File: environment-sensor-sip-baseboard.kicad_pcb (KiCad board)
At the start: 4 copper layers, 50 x 26.5 mm, 60 parts, among them J1 USB-C_GCT_USB4105-GF-A, J2 JST_SH_1x4_SM04B-SRSS-TB-LF-SN, J3 JST_SH_1x4_SM04B-SRSS-TB-LF-SN, U1 Antmicro_GEM3, U5 SHT45, U6 BME280

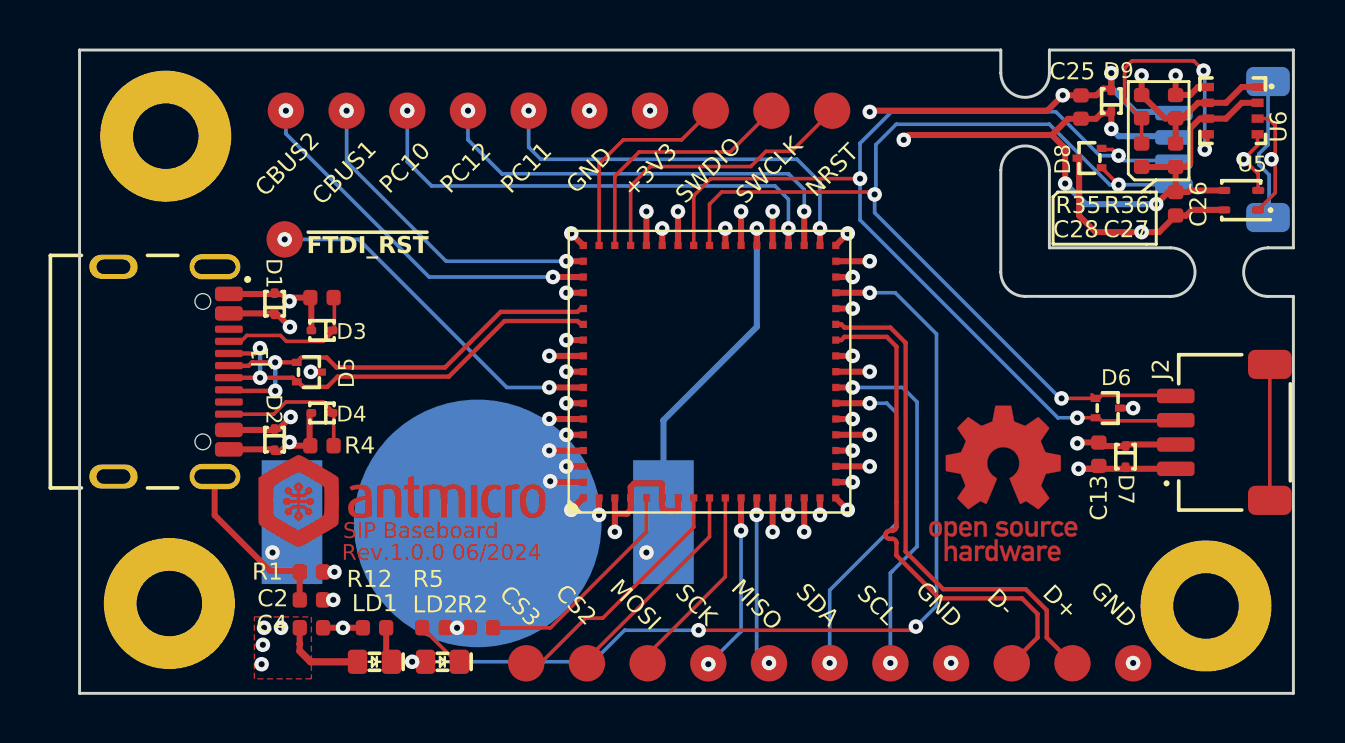
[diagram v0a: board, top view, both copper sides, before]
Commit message: [#61553] Update title block
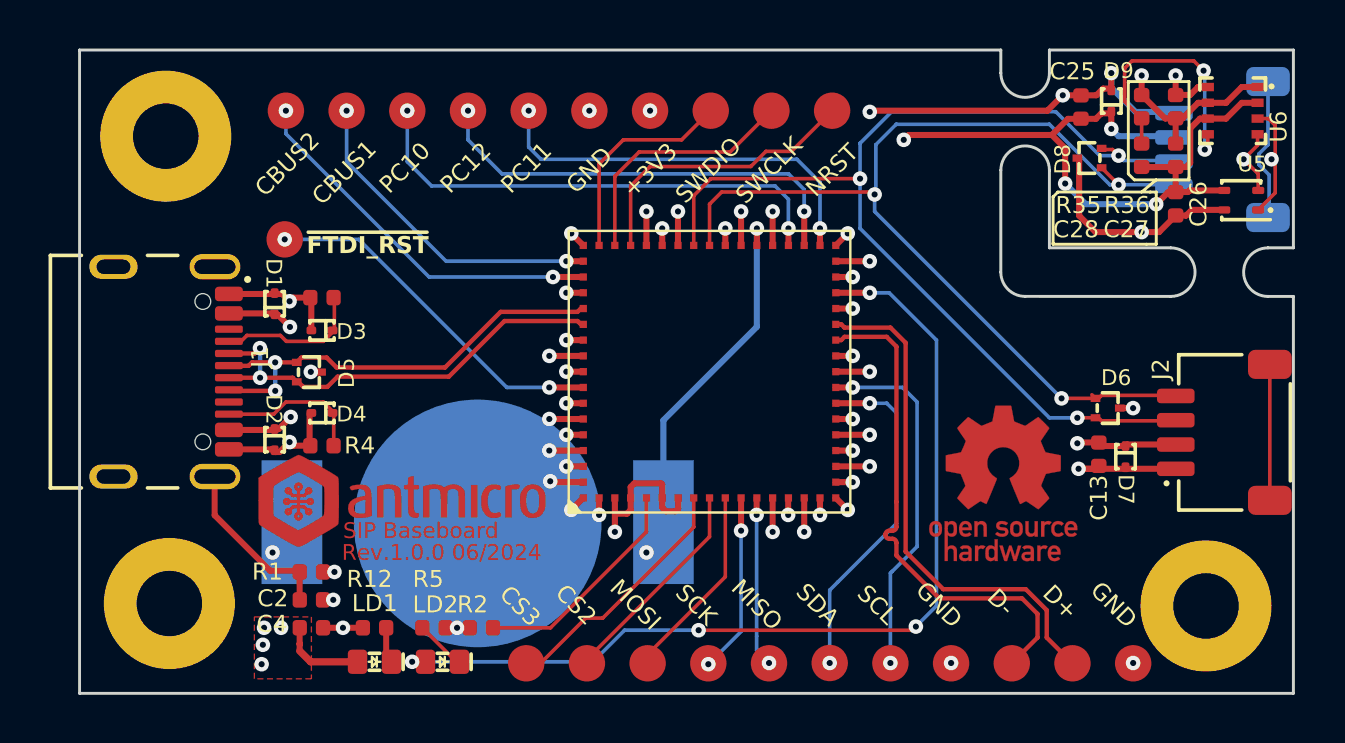
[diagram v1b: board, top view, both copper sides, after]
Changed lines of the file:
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@@
   )
   (paper "A4")
+  (title_block
+    (title "SiP Baseboard")
+    (date "2024-06-28")
+    (rev "1.0.0")
+    (company "Antmicro ")
+    (comment 1 "www.antmicro.com")
+  )
   (layers
     (0 "F.Cu" signal)
@@
     (tags "resistor SMD 0402")
     (property "Author" "Antmicro")
-    (property "DNP" "DNP")
     (property "License" "Apache-2.0")
     (property "MPN" "CR0402-FX-5101GLF")
@@
     (property "ki_description" "SMD Chip Resistor, 5.1 kohm, ± 1%, 63 mW, 0402 [1005 Metric], Thick Film, General Purpose")
     (property "ki_keywords" "0402, SMT, RESISTOR, PASSIVE")
-    (attr smd exclude_from_pos_files exclude_from_bom)
+    (attr smd)
     (fp_text reference "R2" (at -1 -0.55) (layer "F.SilkS")
         (effects (font (size 0.7 0.7) (thickness 0.15)) (justify left bottom))
@@
     (property "ki_description" "SMD Chip Resistor, 100 kohm, ± 1%, 62.5 mW, 0402 [1005 Metric], Thick Film, General Purpose")
     (property "ki_keywords" "0402, SMT, RESISTOR, PASSIVE")
-    (attr smd exclude_from_pos_files exclude_from_bom)
+    (attr smd)
     (fp_text reference "R35" (at -2.465 -3.55 180) (layer "F.SilkS")
         (effects (font (size 0.7 0.7) (thickness 0.15)) (justify left bottom))
@@
     (property "ki_description" "SMD Chip Resistor, 1 Mohm, ± 1%, 62.5 mW, 0402 [1005 Metric], Thick Film, General Purpose")
     (property "ki_keywords" "0402, SMT, RESISTOR, PASSIVE")
-    (attr smd exclude_from_pos_files exclude_from_bom)
+    (attr smd)
     (fp_text reference "R1" (at -2.45 0.4) (layer "F.SilkS")
         (effects (font (size 0.7 0.7) (thickness 0.15)) (justify left bottom))
@@
   (segment (start 207.825 118.125) (end 203.725 118.125) (width 0.15) (layer "In2.Cu") (net 9))
   (segment (start 203.725 118.125) (end 202.8 119.05) (width 0.15) (layer "In2.Cu") (net 9))
+  (segment (start 192.75 119.45) (end 192.75 120.15) (width 0.15) (layer "B.Cu") (net 9))
   (segment (start 193.642 116.558) (end 199.947 116.558) (width 0.15) (layer "B.Cu") (net 9))
-  (segment (start 192.75 119.45) (end 192.75 120.2) (width 0.15) (layer "B.Cu") (net 9))
   (segment (start 202.8 119.05) (end 204.8 119.05) (width 0.15) (layer "B.Cu") (net 9))
   (segment (start 192.8 117.4) (end 193.642 116.558) (width 0.15) (layer "B.Cu") (net 9))
   (segment (start 192.75 119.45) (end 192.8 119.4) (width 0.15) (layer "B.Cu") (net 9))
+  (segment (start 192.75 120.15) (end 200.45 127.85) (width 0.15) (layer "B.Cu") (net 9))
   (segment (start 202.439 119.05) (end 202.8 119.05) (width 0.15) (layer "B.Cu") (net 9))
   (segment (start 192.8 119.4) (end 192.8 117.4) (width 0.15) (layer "B.Cu") (net 9))
-  (segment (start 200.4 127.85) (end 200.45 127.85) (width 0.15) (layer "B.Cu") (net 9))
   (segment (start 199.947 116.558) (end 202.439 119.05) (width 0.15) (layer "B.Cu") (net 9))
-  (segment (start 192.75 120.2) (end 200.4 127.85) (width 0.15) (layer "B.Cu") (net 9))
   (segment (start 185.3 119.5) (end 186 118.8) (width 0.15) (layer "F.Cu") (net 10))
   (segment (start 202.025 117.6) (end 202.55 117.6) (width 0.15) (layer "F.Cu") (net 10))
@@
   (segment (start 209.1 118) (end 208.175 117.075) (width 0.15) (layer "In2.Cu") (net 10))
   (segment (start 203 118.05) (end 204.8 118.05) (width 0.15) (layer "B.Cu") (net 10))
+  (segment (start 192.15 120.85) (end 199.95 128.65) (width 0.15) (layer "B.Cu") (net 10))
   (segment (start 193.449463 116.043) (end 200.214 116.043) (width 0.15) (layer "B.Cu") (net 10))
   (segment (start 200.214 116.043) (end 202.021 117.85) (width 0.15) (layer "B.Cu") (net 10))
   (segment (start 192.15 117.342463) (end 193.449463 116.043) (width 0.15) (layer "B.Cu") (net 10))
   (segment (start 202.021 117.85) (end 202.8 117.85) (width 0.15) (layer "B.Cu") (net 10))
-  (segment (start 192.15 120.5) (end 200.3 128.65) (width 0.15) (layer "B.Cu") (net 10))
+  (segment (start 192.15 118.8) (end 192.15 120.85) (width 0.15) (layer "B.Cu") (net 10))
   (segment (start 202.8 117.85) (end 203 118.05) (width 0.15) (layer "B.Cu") (net 10))
   (segment (start 192.15 118.8) (end 192.15 117.342463) (width 0.15) (layer "B.Cu") (net 10))
-  (segment (start 192.15 118.8) (end 192.15 120.5) (width 0.15) (layer "B.Cu") (net 10))
-  (segment (start 200.3 128.65) (end 201.1 128.65) (width 0.15) (layer "B.Cu") (net 10))
+  (segment (start 199.95 128.65) (end 201.1 128.65) (width 0.15) (layer "B.Cu") (net 10))
   (segment (start 191.15 123.5) (end 192.549999 123.5) (width 0.25) (layer "F.Cu") (net 11))
   (segment (start 194.3 137.4) (end 185.5 137.4) (width 0.15) (layer "F.Cu") (net 11))
@@
   (segment (start 173.7 138.7) (end 181.15 138.7) (width 0.15) (layer "B.Cu") (net 11))
   (segment (start 182.45 137.4) (end 185.5 137.4) (width 0.15) (layer "B.Cu") (net 11))
-  (segment (start 193.6 123.5) (end 192.549999 123.5) (width 0.15) (layer "B.Cu") (net 11))
-  (segment (start 195.3 125.2) (end 193.6 123.5) (width 0.15) (layer "B.Cu") (net 11))
+  (segment (start 195.3 136.4) (end 195.3 125.45) (width 0.15) (layer "B.Cu") (net 11))
   (segment (start 194.45 137.25) (end 195.3 136.4) (width 0.15) (layer "B.Cu") (net 11))
   (segment (start 181.15 138.7) (end 182.45 137.4) (width 0.15) (layer "B.Cu") (net 11))
-  (segment (start 195.3 136.4) (end 195.3 125.2) (width 0.15) (layer "B.Cu") (net 11))
+  (segment (start 195.3 125.45) (end 193.35 123.5) (width 0.15) (layer "B.Cu") (net 11))
+  (segment (start 193.35 123.5) (end 192.549999 123.5) (width 0.15) (layer "B.Cu") (net 11))
   (segment (start 180.75 127.4) (end 179.35 127.4) (width 0.25) (layer "F.Cu") (net 15))
   (via (at 179.35 127.4) (size 0.6) (drill 0.25) (layers "F.Cu" "B.Cu") (net 15))
